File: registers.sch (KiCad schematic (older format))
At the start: 19 parts

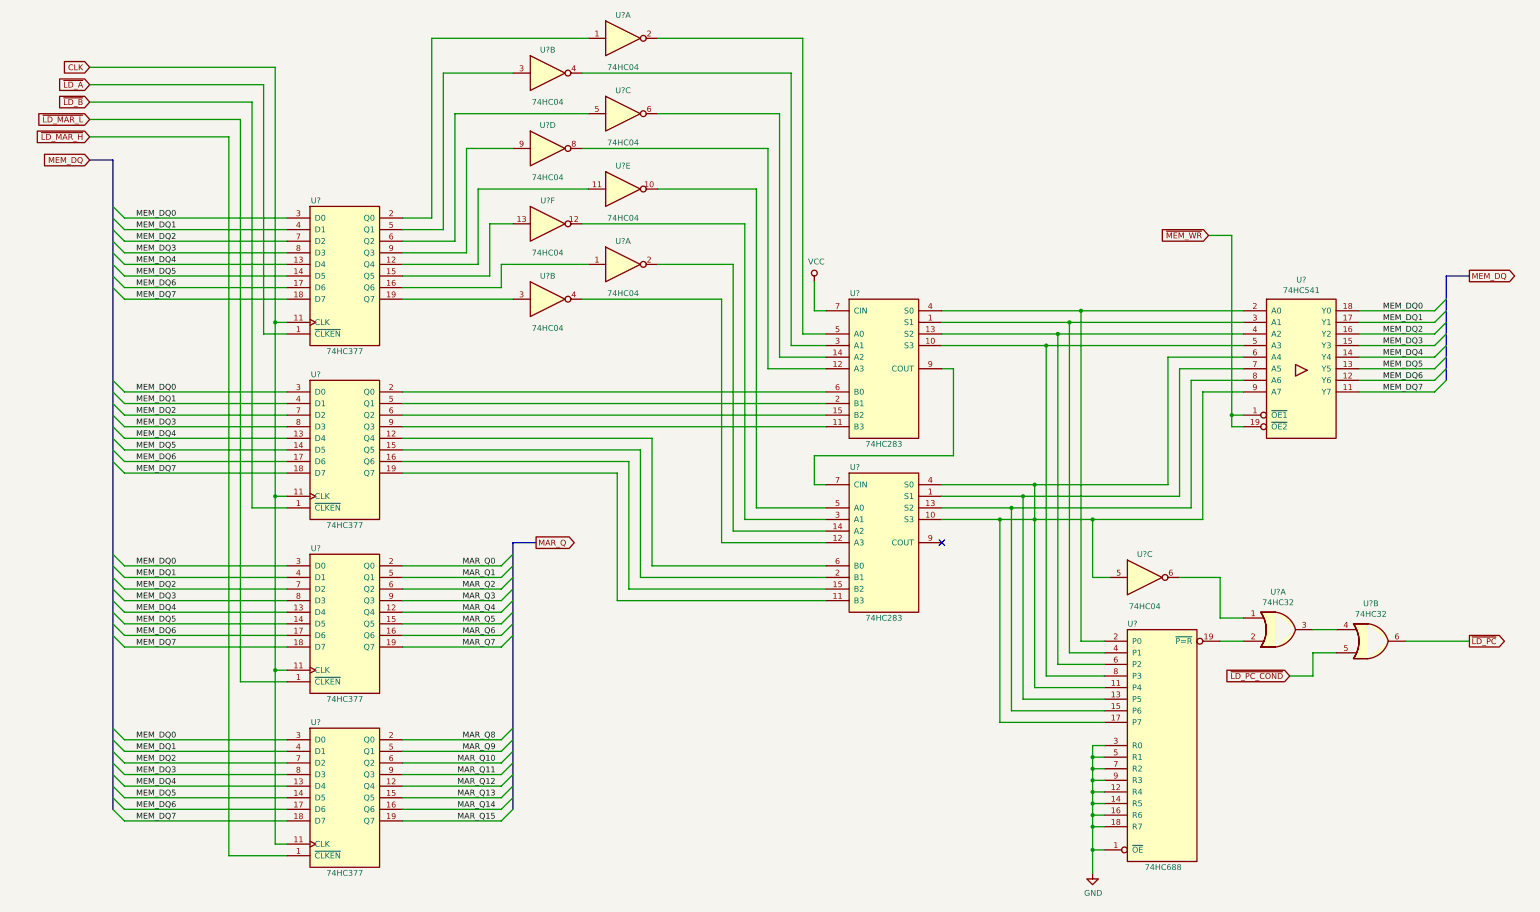
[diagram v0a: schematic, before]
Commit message: backup before registers alu split
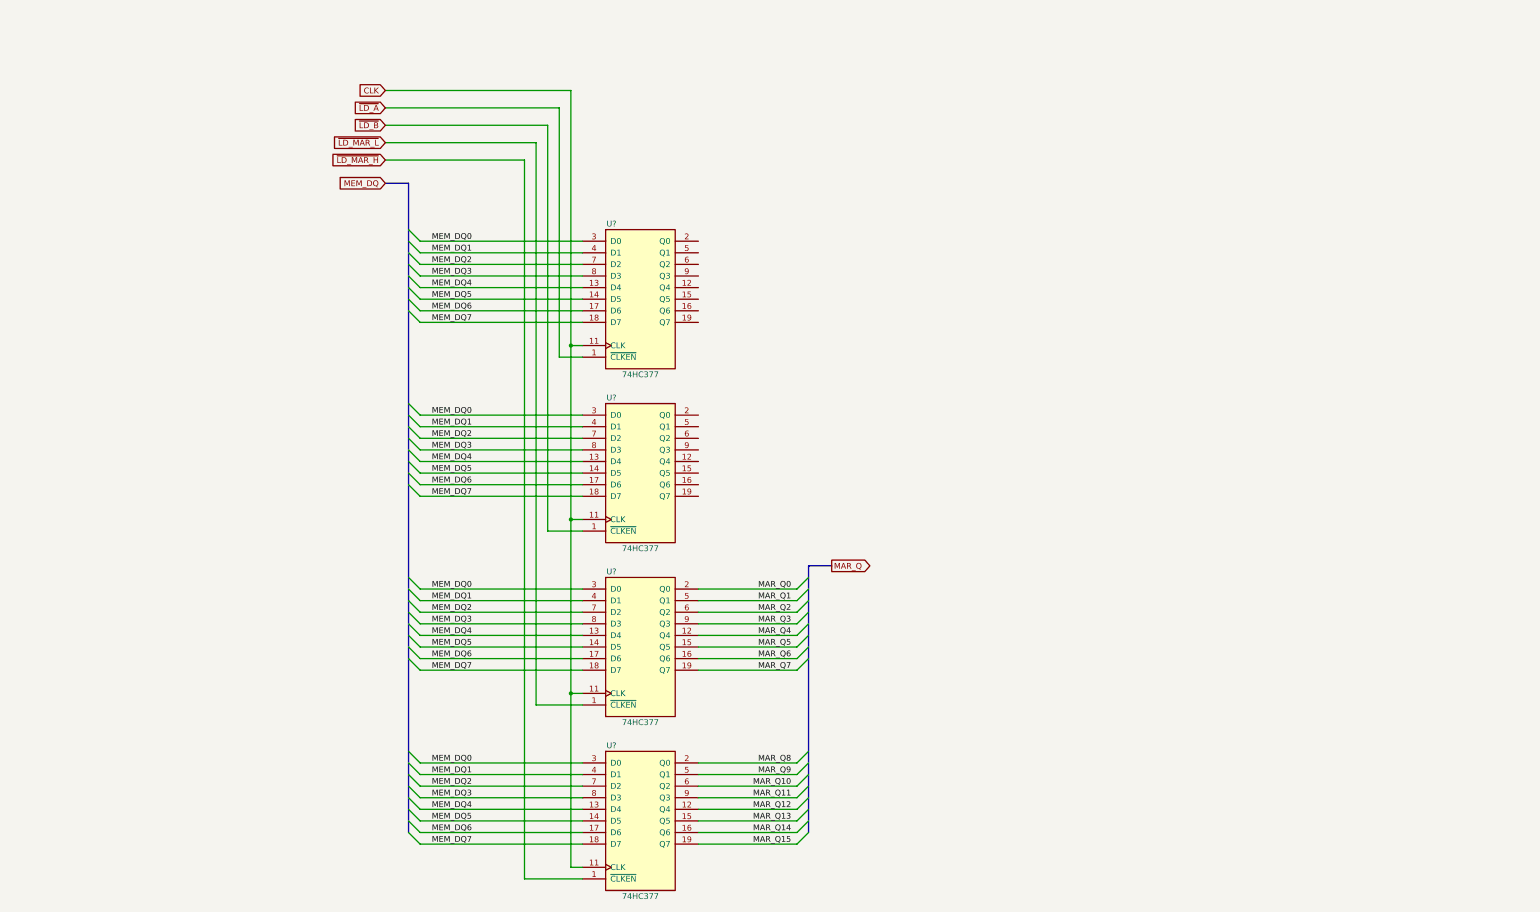
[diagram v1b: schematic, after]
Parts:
- removed U? (x4): 74HC377, symbol 74xx_modified:74LS377
- removed U? (x2): 74HC283, symbol 74xx_modified:74LS283
- removed U? (x9): 74HC04, Package_DIP:DIP-14_W7.62mm, symbol 74xx:74LS04
- removed U?: 74HC688, symbol 74xx_modified:74LS688
- removed U? (x2): 74HC32, symbol 74xx_modified:74LS32
- removed U?: 74HC541, symbol 74xx_modified:74LS541
- added U? (x4): 74HC377, symbol 74xx_modified:74LS377
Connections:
- net CLK: now also U?.11 (CLK), U?.11 (CLK), U?.11 (CLK), U?.11 (CLK)
- net GND: now also U?.10 (GND), U?.10 (GND), U?.10 (GND), U?.10 (GND)
- net MAR_Q0: now also U?.2 (Q0)
- net MAR_Q1: now also U?.5 (Q1)
- net MAR_Q10: now also U?.6 (Q2)
- net MAR_Q11: now also U?.9 (Q3)
- net MAR_Q12: now also U?.12 (Q4)
- net MAR_Q13: now also U?.15 (Q5)
- net MAR_Q14: now also U?.16 (Q6)
- net MAR_Q15: now also U?.19 (Q7)
- net MAR_Q2: now also U?.6 (Q2)
- net MAR_Q3: now also U?.9 (Q3)
- net MAR_Q4: now also U?.12 (Q4)
- net MAR_Q5: now also U?.15 (Q5)
- net MAR_Q6: now also U?.16 (Q6)
- net MAR_Q7: now also U?.19 (Q7)
- net MAR_Q8: now also U?.2 (Q0)
- net MAR_Q9: now also U?.5 (Q1)
- net MEM_DQ0: now also U?.3 (D0), U?.3 (D0), U?.3 (D0), U?.3 (D0)
- net MEM_DQ1: now also U?.4 (D1), U?.4 (D1), U?.4 (D1), U?.4 (D1)
- net MEM_DQ2: now also U?.7 (D2), U?.7 (D2), U?.7 (D2), U?.7 (D2)
- net MEM_DQ3: now also U?.8 (D3), U?.8 (D3), U?.8 (D3), U?.8 (D3)
- net MEM_DQ4: now also U?.13 (D4), U?.13 (D4), U?.13 (D4), U?.13 (D4)
- net MEM_DQ5: now also U?.14 (D5), U?.14 (D5), U?.14 (D5), U?.14 (D5)
- net MEM_DQ6: now also U?.17 (D6), U?.17 (D6), U?.17 (D6), U?.17 (D6)
- net MEM_DQ7: now also U?.18 (D7), U?.18 (D7), U?.18 (D7), U?.18 (D7)
- net VCC: now also U?.20 (VCC), U?.20 (VCC), U?.20 (VCC), U?.20 (VCC)
- net ~LD_A: now also U?.1 (~CLKEN)
- net ~LD_B: now also U?.1 (~CLKEN)
- net ~LD_MAR_H: now also U?.1 (~CLKEN)
- net ~LD_MAR_L: now also U?.1 (~CLKEN)
- no-connect marks 1 -> 0
